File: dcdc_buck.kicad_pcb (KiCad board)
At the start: 2 copper layers, 100 x 60 mm, 79 parts, among them J3 Conn_01x02_Socket, J4 Conn_01x02_Socket, Q11 MMBT3904, Q12 MMBT3906, Q13 MMBT3904, Q5 IRF9Z24N, Q6 MMBT3904, U1 TLV9151DBV, U2 TLV9151DBV, U3 TLV9151DBV, U4 TL431DBV, U6 INA241B4IDR

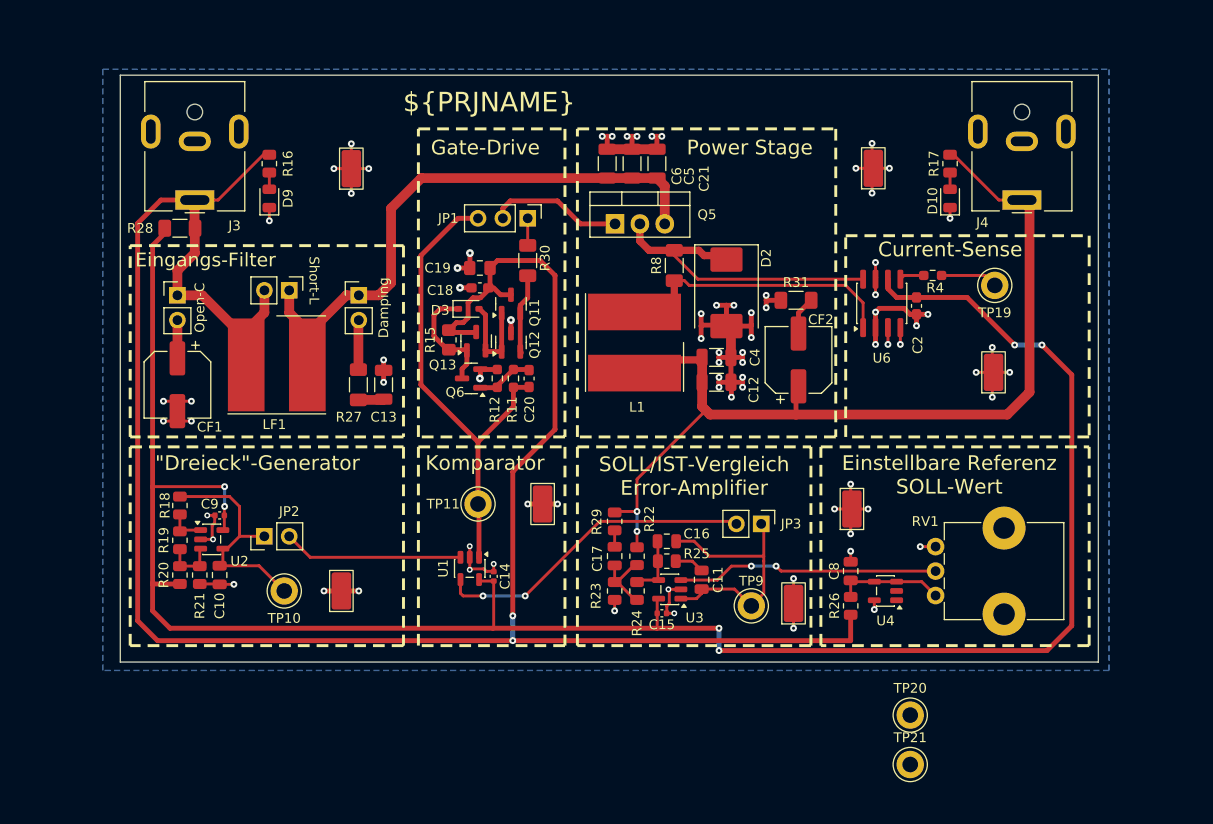
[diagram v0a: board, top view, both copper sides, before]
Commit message: made room for Version 1.1 (WiP)
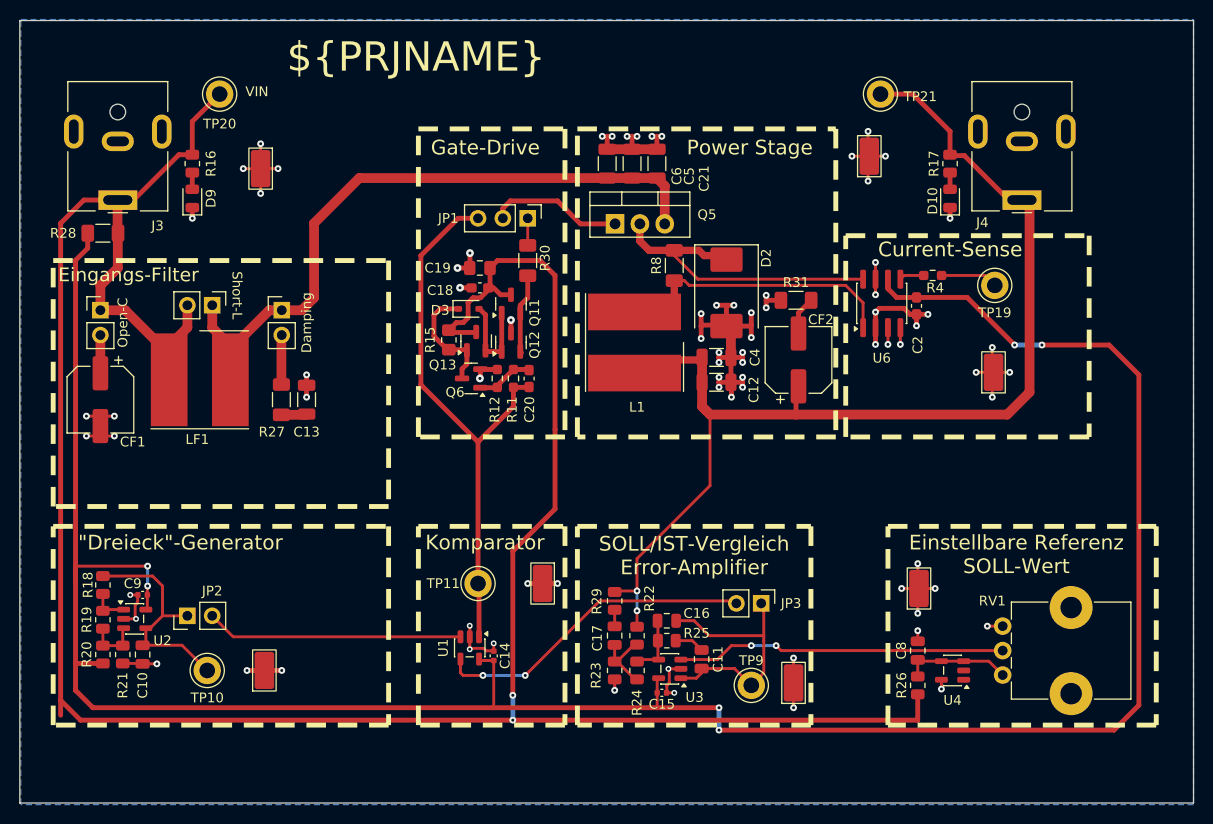
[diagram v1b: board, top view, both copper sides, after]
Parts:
- moved TP20 95.0 mm to (100.6, 74.2)
- moved TP21 68.6 mm to (168.1, 74.2)
- moved C10 11.3 mm to (92.7, 131.5)
- moved C9 11.3 mm to (92.7, 125.4)
- moved JP2 11.3 mm to (97.3, 127.5)
- moved R21 11.3 mm to (90.7, 131.5)
- moved TP10 11.3 mm to (99.3, 133.1)
- moved R18 11.3 mm to (88.6, 124.4)
- moved R19 11.3 mm to (88.6, 127.9)
- moved R20 11.3 mm to (88.6, 131.5)
- moved TP16 11.3 mm to (105.2, 133.1)
- moved U2 11.3 mm to (91.9, 127.8)
- moved R26 10.6 mm to (172.0, 134.6)
- moved TP13 10.6 mm to (172.1, 124.7)
- moved U4 10.6 mm to (175.5, 133.1)
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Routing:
- net VIN: track 224.9 -> 266.3 mm
- net VCC: track 211.0 -> 250.3 mm
- net VOUT: track 98.8 -> 117.8 mm
- net Net-(JP4-A): track 59.9 -> 68.4 mm
- net /PP_IN: track 49.4 -> 57.6 mm
- net /Dreieck_Komp: track 18.4 -> 26.3 mm
- net Net-(U3-+): track 26.8 -> 33.7 mm
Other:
- board size 100 x 60 mm -> 120 x 80 mm
- board text added: "Franz Patz Juli 2026"
- board text added: "VIN"
- board text removed: "Franz Patz Juni 2026"
